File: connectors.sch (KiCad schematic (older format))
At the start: 7 parts, among them J1 Wuerth_7499010121A, J4 Micro_SD_Card, U2 ET60T-02-24-02-X-RTX-GP

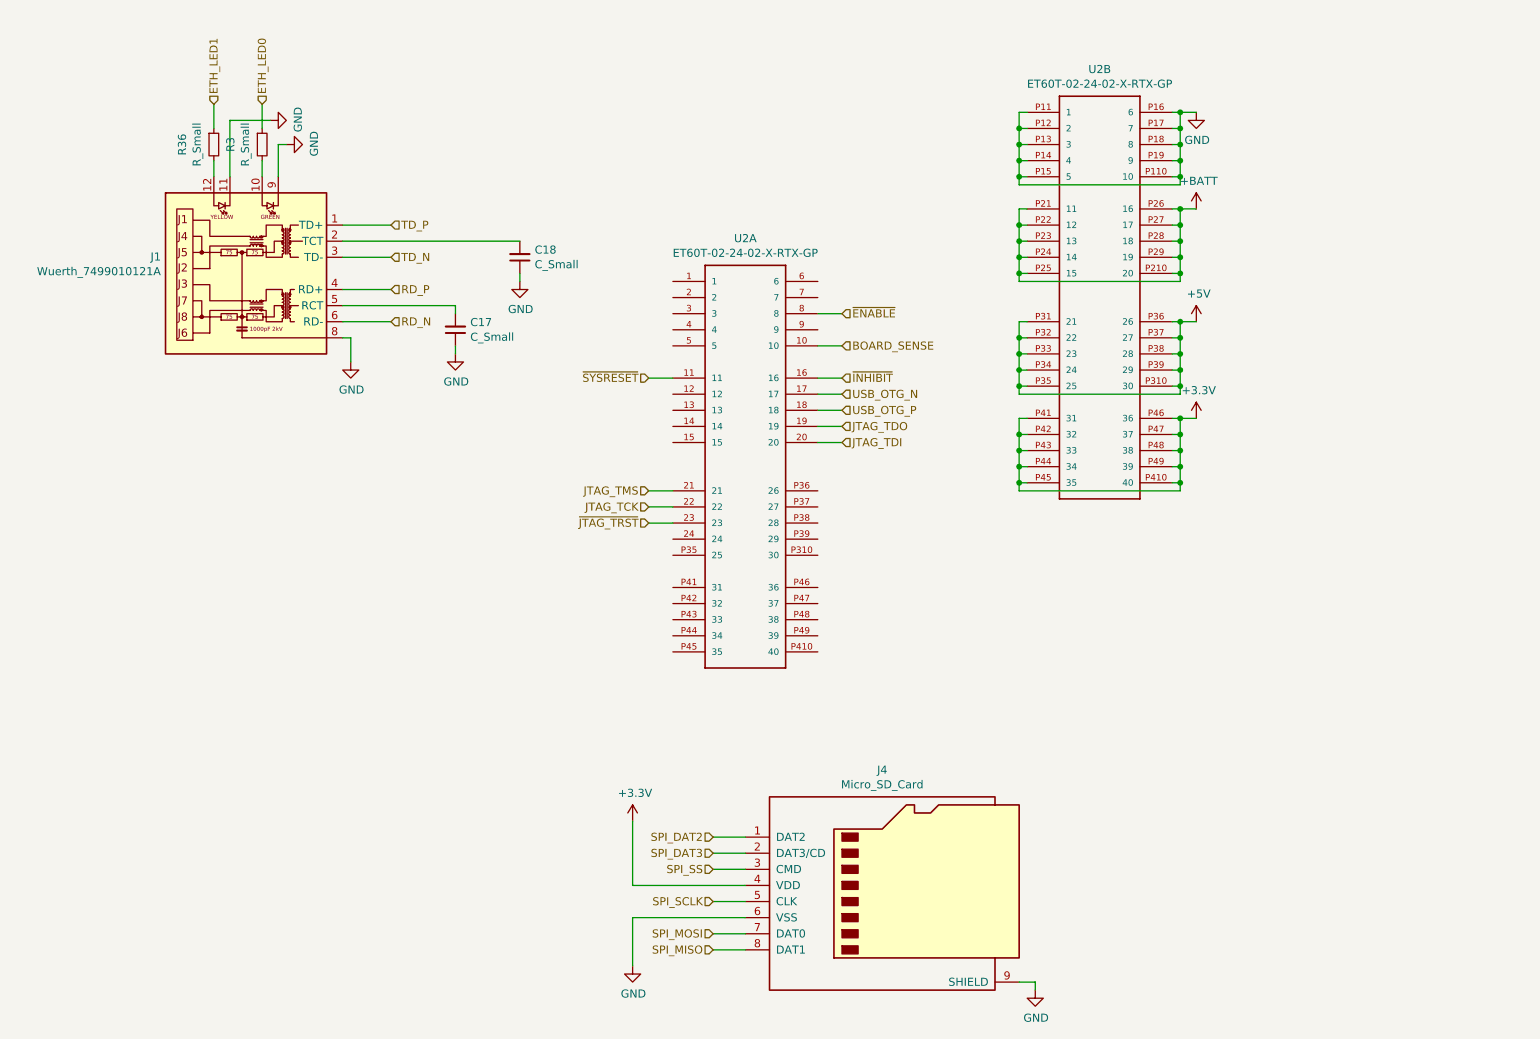
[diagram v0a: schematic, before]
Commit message: updates
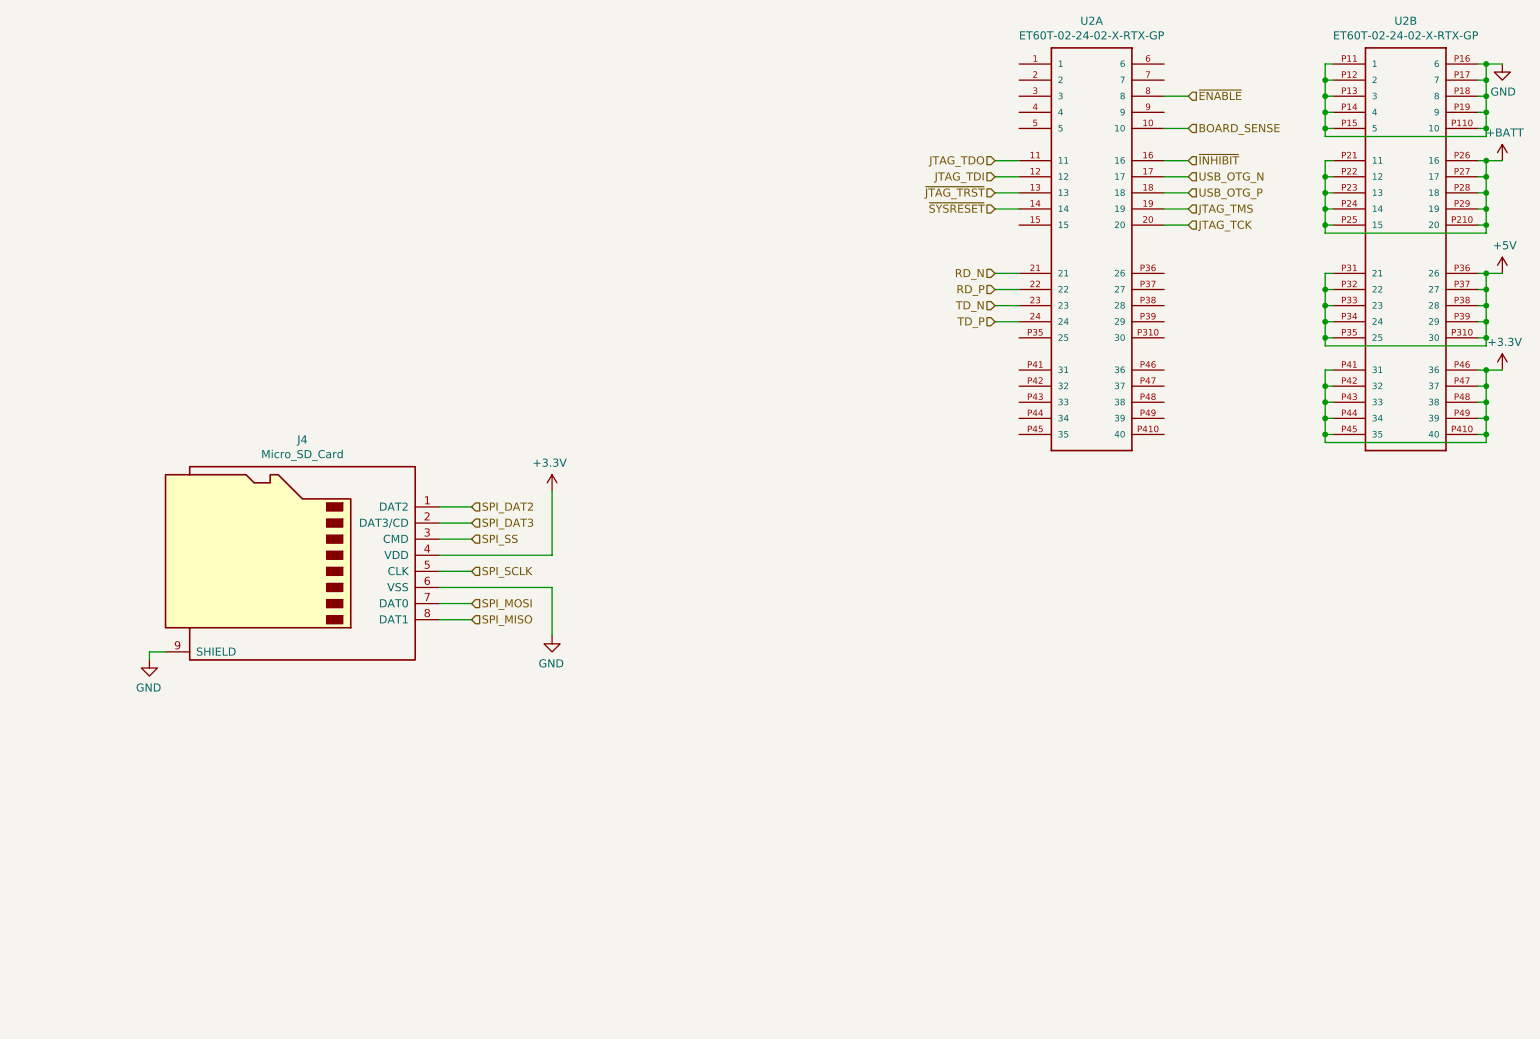
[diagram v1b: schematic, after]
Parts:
- removed C17, C18: C_Small, Capacitor_SMD:C_0603_1608Metric, symbol Device:C_Small
- removed J1: Wuerth_7499010121A, Connector_RJ:RJ45_Wuerth_7499010121A_Horizontal, symbol Connector:Wuerth_7499010121A
- removed R3: R_Small, symbol Device:R_Small
- removed R36: R_Small, Resistor_SMD:R_0603_1608Metric, symbol Device:R_Small
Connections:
- net JTAG_TCK: now also U2.20; no longer U2.22
- net JTAG_TDI: now also U2.12; no longer U2.20
- net JTAG_TDO: now also U2.11; no longer U2.19
- net JTAG_TMS: now also U2.19; no longer U2.21
- net RD_N: now also U2.21
- net RD_P: now also U2.22
- net TD_N: now also U2.23
- net TD_P: now also U2.24
- net ~JTAG_TRST: now also U2.13; no longer U2.23
- net ~SYSRESET: now also U2.14; no longer U2.11
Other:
- moved on the sheet: J4, U2A, U2B
